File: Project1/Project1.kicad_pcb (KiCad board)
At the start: 2 copper layers, 83.8 x 99.1 mm, 37 parts, among them J1 Conn_01x03_Female, J2 Conn_01x02_Male, SW1 SW_DP3T, SW2 SW_DPDT_x2, U1 LM324, U2 LM324, U3 NE555P

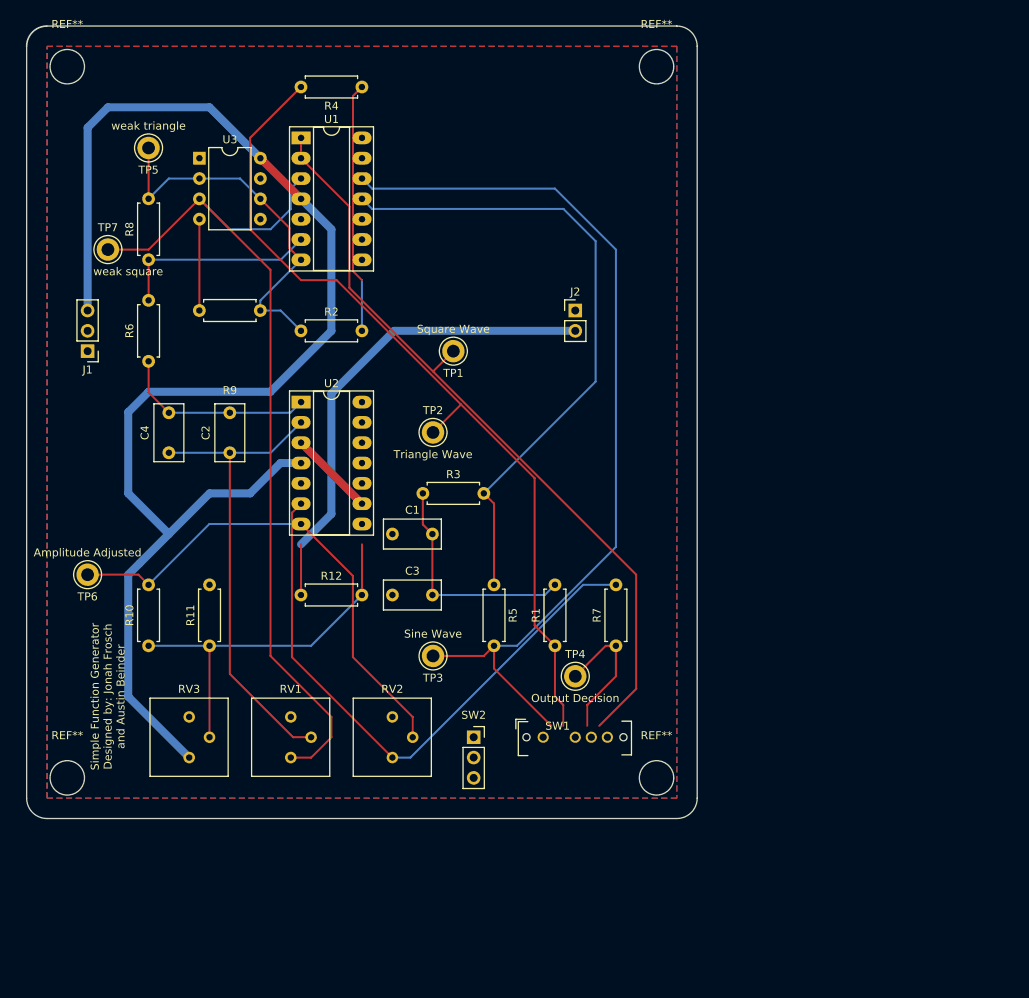
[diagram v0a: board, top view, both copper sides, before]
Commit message: redesigned board
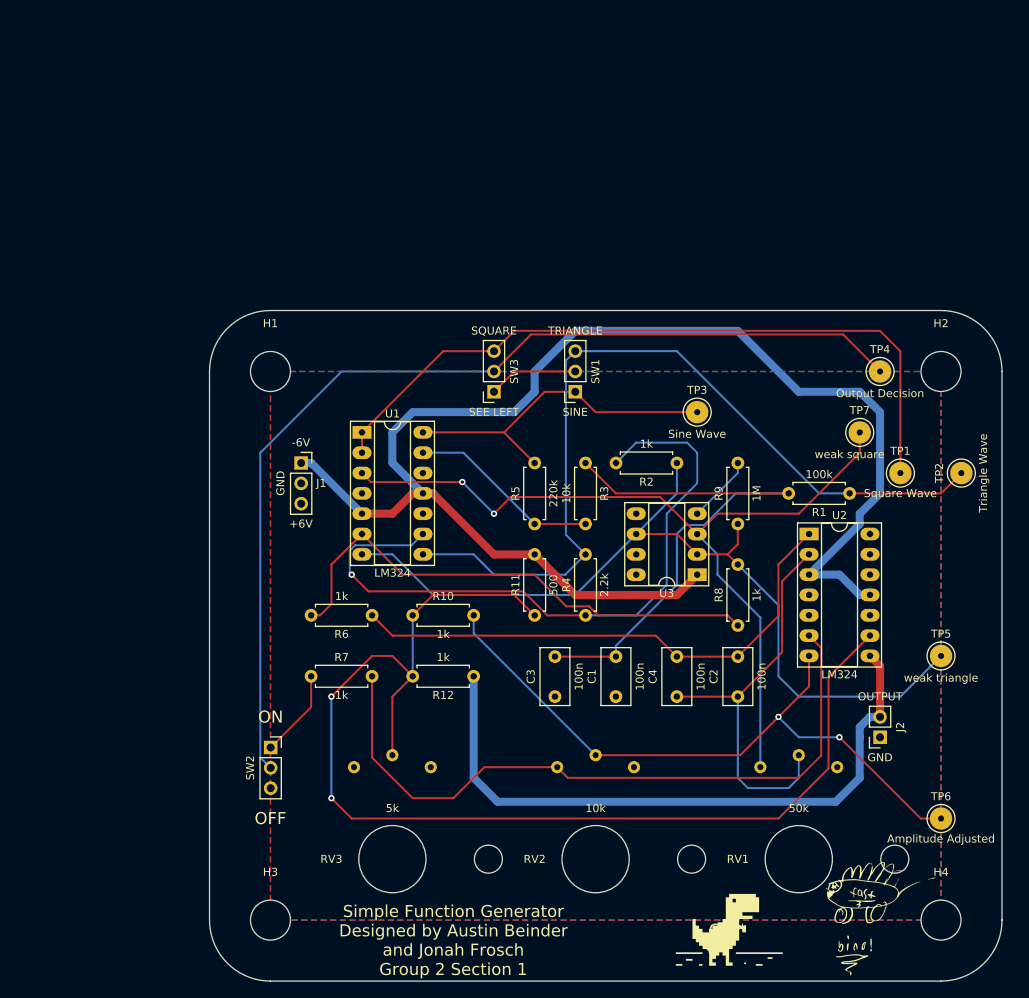
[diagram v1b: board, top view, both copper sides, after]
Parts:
- removed REF** (x4): MountingHole_4.3mm_M4, MountingHole:MountingHole_4.3mm_M4
- added G***: LOGO, LOGO, F.Cu at (166.4, 148.6)
- added G***: LOGO, LOGO, F.Cu at (185.4, 147.3)
- added H1: MountingHole, MountingHole:MountingHole_5mm, F.Cu at (109.2, 78.7)
- added H2: MountingHole, MountingHole:MountingHole_5mm, F.Cu at (193.0, 78.7)
- added H3: MountingHole, MountingHole:MountingHole_5mm, F.Cu at (109.2, 147.3)
- added H4: MountingHole, MountingHole:MountingHole_5mm, F.Cu at (193.0, 147.3)
- added SW3: SW_DPDT_x2, Connector_PinSocket_2.54mm:PinSocket_1x03_P2.54mm_Vertical, F.Cu at (137.2, 81.3)
- J1: footprint Connector_PinHeader_2.54mm:PinHeader_1x03_P2.54mm_Vertical -> Connector_PinSocket_2.54mm:PinSocket_1x03_P2.54mm_Vertical
- J2: footprint Connector_PinHeader_2.54mm:PinHeader_1x02_P2.54mm_Vertical -> Connector_PinSocket_2.54mm:PinSocket_1x02_P2.54mm_Vertical
- R1: value 2.5k -> 100k
- R3: value 2.5k -> 10k
- R4: value 2.5k -> 2.2k
- R5: value 250k -> 220k
- RV1, RV2, RV3: footprint Potentiometer_THT:Potentiometer_Bourns_3386P_Vertical -> custom:Chomkypot
- SW1: value SW_DP3T -> SW_DPDT_x2; footprint Switches:SW_SP3T -> Connector_PinSocket_2.54mm:PinSocket_1x03_P2.54mm_Vertical
- U3: footprint Package_DIP:DIP-8_W7.62mm -> Package_DIP:DIP-8_W7.62mm_Socket_LongPads
- moved TP5 117.7 mm to (193.0, 114.3), turned to 0 degrees
- moved TP6 110.9 mm to (193.0, 134.6), turned to 0 degrees
- moved TP7 96.7 mm to (182.9, 86.4)
- moved R8 86.7 mm to (167.6, 110.5)
- moved U3 81.1 mm to (162.6, 104.1), turned to 180 degrees
- moved R4 71.7 mm to (148.6, 109.2), turned to 90 degrees
- moved C4 70.4 mm to (160.0, 119.4)
- moved C2 70.4 mm to (167.6, 119.4)
- moved TP2 66.2 mm to (195.6, 91.4), turned to 90 degrees
- moved U2 65.6 mm to (176.5, 99.1)
- moved J2 65.5 mm to (185.4, 124.5), turned to 180 degrees
- moved R9 65.4 mm to (167.6, 97.8), turned to 90 degrees
- moved RV1 64.8 mm to (175.3, 139.7)
- moved TP1 57.9 mm to (188.0, 91.4), turned to 0 degrees
- moved TP4 53.9 mm to (185.4, 78.7)
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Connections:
- SW1 pad 2: triangle_wave -> Net-(SW1-Pad2)
- SW1 pad 3: Net-(SW1-Pad3) -> triangle_wave
- SW2 pad 2: Net-(SW1-Pad3) -> Net-(SW2-Pad2)
- TP4 pad 1: Net-(SW1-Pad3) -> Net-(SW2-Pad2)
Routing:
- net +6V: track 286.5 -> 0.00 mm
- net Net-(R3-Pad2): track 219.8 -> 24.0 mm
- net -6V: track 10.8 -> 173.3 mm
- net Net-(SW2-Pad2): track 0.00 -> 125.4 mm
- net square_wave_weak: track 0.00 -> 106.3 mm, vias 0 -> 2
- net Net-(R10-Pad1): track 47.1 -> 146.4 mm, vias 0 -> 2
- net Net-(R7-Pad2): track 0.00 -> 87.3 mm
- net Net-(R2-Pad2): track 6.34 -> 86.0 mm, vias 0 -> 1
- net triangle_weak: track 46.7 -> 108.7 mm
- net Net-(R10-Pad2): track 137.1 -> 83.4 mm, vias 0 -> 2
- net sine_wave: track 0.00 -> 42.8 mm
- net Net-(C2-Pad2): track 24.6 -> 66.9 mm
- net Net-(C1-Pad2): track 29.0 -> 69.1 mm
- net Net-(R6-Pad2): track 25.2 -> 65.2 mm
- net output_waveform: track 60.5 -> 81.0 mm
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- added copper zone on F.Cu, net +6V
- added copper zone on B.Cu, net GND
- removed copper zone on B.Cu, net -6V
- removed copper zone on F.Cu, net GND
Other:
- board size 83.8 x 99.1 mm -> 99.1 x 83.8 mm
- board text added: "+6V"
- board text added: "-6V"
- board text added: "10k"
- board text added: "50k"
- board text added: "5k"
- board text added: "GND"
- board text added: "OFF"
- board text added: "ON"
- board text added: "OUTPUT"
- board text added: "SEE LEFT"
- board text added: "SINE"
- board text added: "SQUARE"
- board text added: "Simple Function Generator Designed by Austin Beinder and Jonah Frosch Group 2 Section 1"
- board text added: "TRIANGLE"
- board text removed: "Simple Function Generator Designed by: Jonah Frosch and Austin Beinder"
